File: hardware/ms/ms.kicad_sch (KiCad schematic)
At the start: 4 parts, among them U1 TP4056-42-ESOP8, U2 STM32G031G8Ux, U3 Opamp_Dual

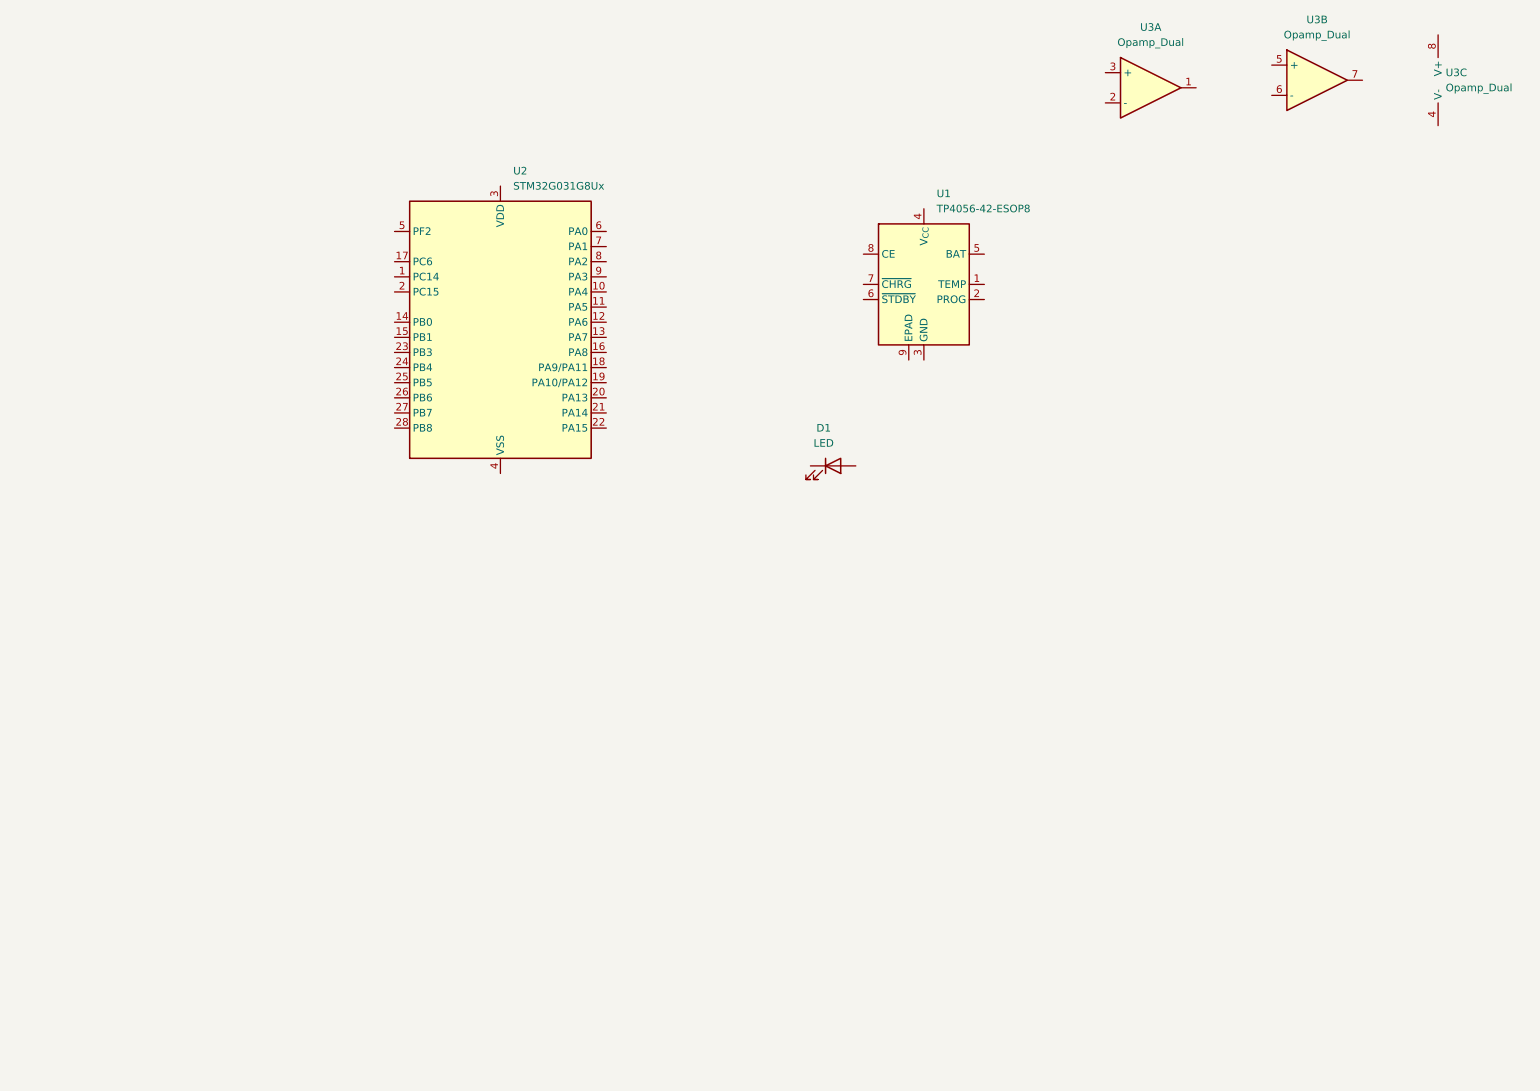
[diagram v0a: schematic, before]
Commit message: hardware update
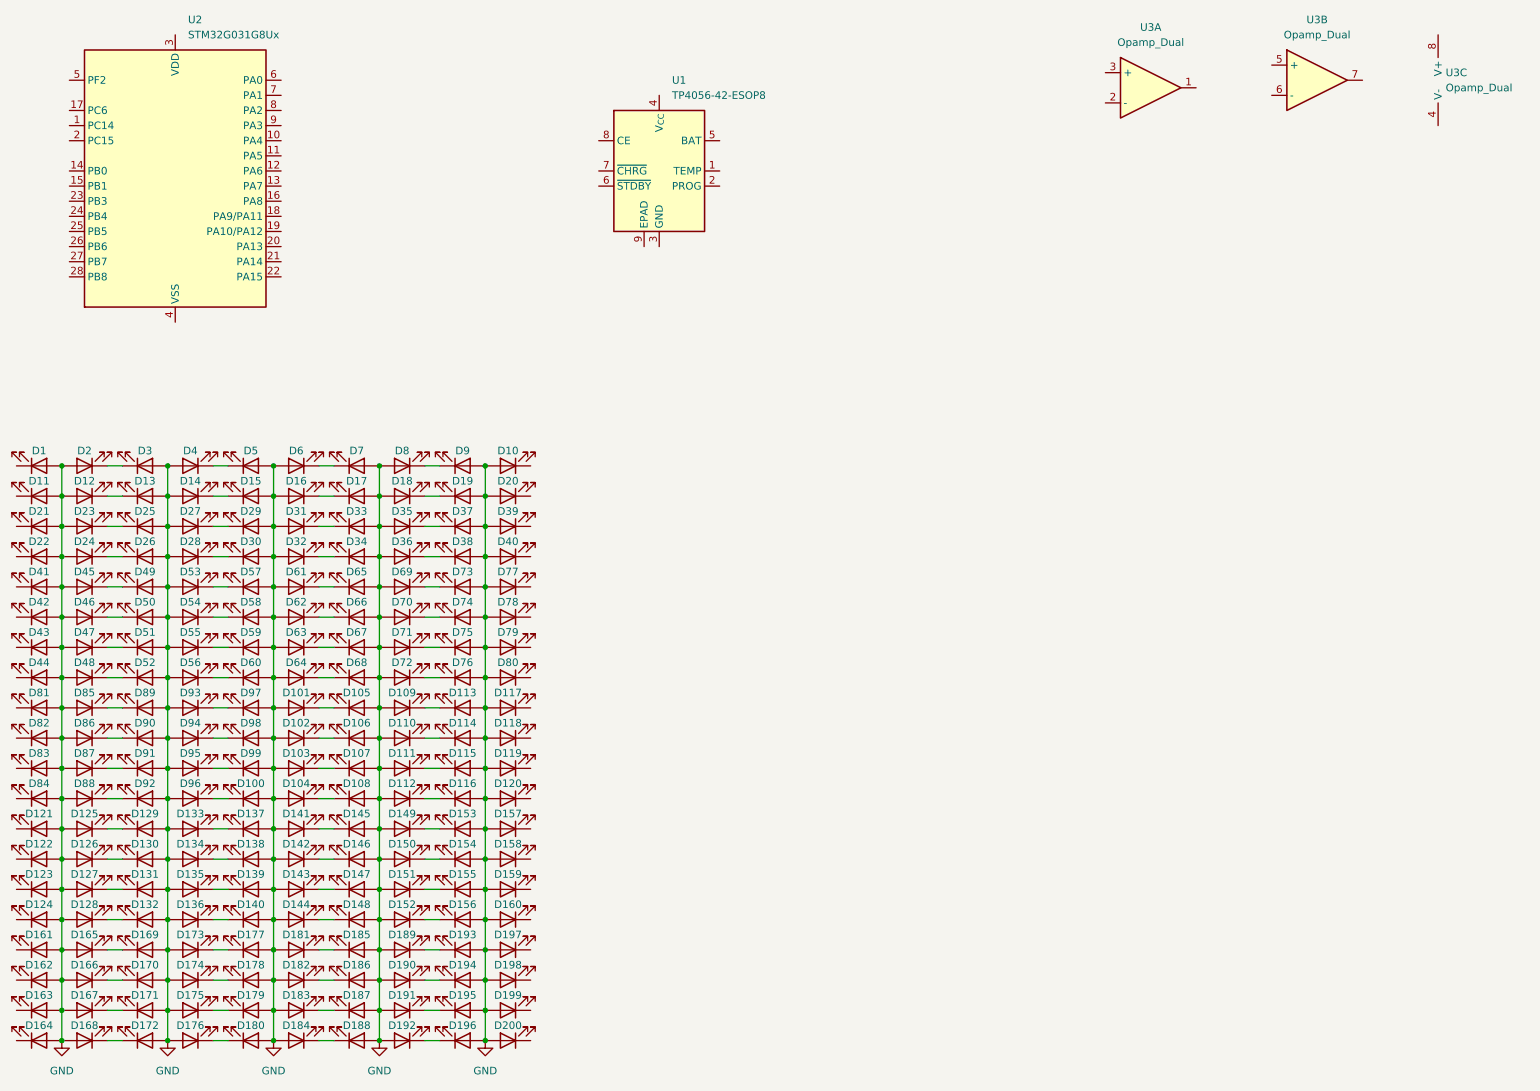
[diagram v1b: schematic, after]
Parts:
- added D10, D100, D101, D102, D103, D104, D105, D106, D107, D108, D109, D11, D110, D111, D112, D113, D114, D115, D116, D117, D118, D119, D12, D120, D121, D122, D123, D124, D125, D126, D127, D128, D129, D13, D130, D131, D132, D133, D134, D135, D136, D137, D138, D139, D14, D140, D141, D142, D143, D144, D145, D146, D147, D148, D149, D15, D150, D151, D152, D153, D154, D155, D156, D157, D158, D159, D16, D160, D161, D162, D163, D164, D165, D166, D167, D168, D169, D17, D170, D171, D172, D173, D174, D175, D176, D177, D178, D179, D18, D180, D181, D182, D183, D184, D185, D186, D187, D188, D189, D19, D190, D191, D192, D193, D194, D195, D196, D197, D198, D199, D2, D20, D200, D21, D22, D23, D24, D25, D26, D27, D28, D29, D3, D30, D31, D32, D33, D34, D35, D36, D37, D38, D39, D4, D40, D41, D42, D43, D44, D45, D46, D47, D48, D49, D5, D50, D51, D52, D53, D54, D55, D56, D57, D58, D59, D6, D60, D61, D62, D63, D64, D65, D66, D67, D68, D69, D7, D70, D71, D72, D73, D74, D75, D76, D77, D78, D79, D8, D80, D81, D82, D83, D84, D85, D86, D87, D88, D89, D9, D90, D91, D92, D93, D94, D95, D96, D97, D98, D99: LED, Library:LED, symbol Device:LED
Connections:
- net GND: now reaches D1.2 (A)
- net GND: now also D10.2 (A), D100.2 (A), D101.2 (A), D102.2 (A), D103.2 (A), D104.2 (A), D105.2 (A), D106.2 (A), D107.2 (A), D108.2 (A), D109.2 (A), D11.2 (A), D110.2 (A), D111.2 (A), D112.2 (A), D113.2 (A), D114.2 (A), D115.2 (A), D116.2 (A), D117.2 (A), D118.2 (A), D119.2 (A), D12.2 (A), D120.2 (A), D121.2 (A), D122.2 (A), D123.2 (A), D124.2 (A), D125.2 (A), D126.2 (A), D127.2 (A), D128.2 (A), D129.2 (A), D13.2 (A), D130.2 (A), D131.2 (A), D132.2 (A), D133.2 (A), D134.2 (A), D135.2 (A), D136.2 (A), D137.2 (A), D138.2 (A), D139.2 (A), D14.2 (A), D140.2 (A), D141.2 (A), D142.2 (A), D143.2 (A), D144.2 (A), D145.2 (A), D146.2 (A), D147.2 (A), D148.2 (A), D149.2 (A), D15.2 (A), D150.2 (A), D151.2 (A), D152.2 (A), D153.2 (A), D154.2 (A), D155.2 (A), D156.2 (A), D157.2 (A), D158.2 (A), D159.2 (A), D16.2 (A), D160.2 (A), D161.2 (A), D162.2 (A), D163.2 (A), D164.2 (A), D165.2 (A), D166.2 (A), D167.2 (A), D168.2 (A), D169.2 (A), D17.2 (A), D170.2 (A), D171.2 (A), D172.2 (A), D173.2 (A), D174.2 (A), D175.2 (A), D176.2 (A), D177.2 (A), D178.2 (A), D179.2 (A), D18.2 (A), D180.2 (A), D181.2 (A), D182.2 (A), D183.2 (A), D184.2 (A), D185.2 (A), D186.2 (A), D187.2 (A), D188.2 (A), D189.2 (A), D19.2 (A), D190.2 (A), D191.2 (A), D192.2 (A), D193.2 (A), D194.2 (A), D195.2 (A), D196.2 (A), D197.2 (A), D198.2 (A), D199.2 (A), D2.2 (A), D20.2 (A), D200.2 (A), D21.2 (A), D22.2 (A), D23.2 (A), D24.2 (A), D25.2 (A), D26.2 (A), D27.2 (A), D28.2 (A), D29.2 (A), D3.2 (A), D30.2 (A), D31.2 (A), D32.2 (A), D33.2 (A), D34.2 (A), D35.2 (A), D36.2 (A), D37.2 (A), D38.2 (A), D39.2 (A), D4.2 (A), D40.2 (A), D41.2 (A), D42.2 (A), D43.2 (A), D44.2 (A), D45.2 (A), D46.2 (A), D47.2 (A), D48.2 (A), D49.2 (A), D5.2 (A), D50.2 (A), D51.2 (A), D52.2 (A), D53.2 (A), D54.2 (A), D55.2 (A), D56.2 (A), D57.2 (A), D58.2 (A), D59.2 (A), D6.2 (A), D60.2 (A), D61.2 (A), D62.2 (A), D63.2 (A), D64.2 (A), D65.2 (A), D66.2 (A), D67.2 (A), D68.2 (A), D69.2 (A), D7.2 (A), D70.2 (A), D71.2 (A), D72.2 (A), D73.2 (A), D74.2 (A), D75.2 (A), D76.2 (A), D77.2 (A), D78.2 (A), D79.2 (A), D8.2 (A), D80.2 (A), D81.2 (A), D82.2 (A), D83.2 (A), D84.2 (A), D85.2 (A), D86.2 (A), D87.2 (A), D88.2 (A), D89.2 (A), D9.2 (A), D90.2 (A), D91.2 (A), D92.2 (A), D93.2 (A), D94.2 (A), D95.2 (A), D96.2 (A), D97.2 (A), D98.2 (A), D99.2 (A)
- new net: D142.1 (K), D146.1 (K)
- new net: D64.1 (K), D68.1 (K)
- new net: D167.1 (K), D171.1 (K)
- new net: D35.1 (K), D37.1 (K)
- new net: D152.1 (K), D156.1 (K)
- new net: D87.1 (K), D91.1 (K)
- new net: D62.1 (K), D66.1 (K)
- new net: D173.1 (K), D177.1 (K)
- new net: D23.1 (K), D25.1 (K)
- new net: D63.1 (K), D67.1 (K)
- new net: D71.1 (K), D75.1 (K)
- new net: D8.1 (K), D9.1 (K)
- new net: D135.1 (K), D139.1 (K)
- new net: D184.1 (K), D188.1 (K)
- new net: D168.1 (K), D172.1 (K)
- new net: D166.1 (K), D170.1 (K)
- new net: D88.1 (K), D92.1 (K)
- new net: D12.1 (K), D13.1 (K)
- new net: D141.1 (K), D145.1 (K)
- new net: D61.1 (K), D65.1 (K)
- new net: D2.1 (K), D3.1 (K)
- new net: D36.1 (K), D38.1 (K)
- new net: D144.1 (K), D148.1 (K)
- new net: D175.1 (K), D179.1 (K)
- new net: D95.1 (K), D99.1 (K)
- new net: D190.1 (K), D194.1 (K)
- new net: D191.1 (K), D195.1 (K)
- new net: D103.1 (K), D107.1 (K)
- new net: D100.1 (K), D96.1 (K)
- new net: D176.1 (K), D180.1 (K)
- new net: D14.1 (K), D15.1 (K)
- new net: D27.1 (K), D29.1 (K)
- new net: D109.1 (K), D113.1 (K)
- new net: D93.1 (K), D97.1 (K)
- new net: D125.1 (K), D129.1 (K)
- new net: D104.1 (K), D108.1 (K)
- new net: D31.1 (K), D33.1 (K)
- new net: D182.1 (K), D186.1 (K)
- new net: D181.1 (K), D185.1 (K)
- new net: D56.1 (K), D60.1 (K)
- new net: D189.1 (K), D193.1 (K)
- new net: D24.1 (K), D26.1 (K)
- new net: D111.1 (K), D115.1 (K)
- new net: D110.1 (K), D114.1 (K)
- new net: D86.1 (K), D90.1 (K)
- new net: D6.1 (K), D7.1 (K)
- new net: D165.1 (K), D169.1 (K)
- new net: D112.1 (K), D116.1 (K)
- new net: D126.1 (K), D130.1 (K)
- new net: D150.1 (K), D154.1 (K)
- new net: D151.1 (K), D155.1 (K)
- new net: D69.1 (K), D73.1 (K)
- new net: D70.1 (K), D74.1 (K)
- new net: D85.1 (K), D89.1 (K)
- new net: D183.1 (K), D187.1 (K)
- new net: D47.1 (K), D51.1 (K)
- new net: D46.1 (K), D50.1 (K)
- new net: D101.1 (K), D105.1 (K)
- new net: D127.1 (K), D131.1 (K)
- new net: D136.1 (K), D140.1 (K)
- new net: D133.1 (K), D137.1 (K)
- new net: D53.1 (K), D57.1 (K)
- new net: D18.1 (K), D19.1 (K)
- new net: D174.1 (K), D178.1 (K)
- new net: D4.1 (K), D5.1 (K)
- new net: D94.1 (K), D98.1 (K)
- new net: D102.1 (K), D106.1 (K)
- new net: D28.1 (K), D30.1 (K)
- new net: D134.1 (K), D138.1 (K)
- new net: D143.1 (K), D147.1 (K)
- new net: D45.1 (K), D49.1 (K)
- new net: D128.1 (K), D132.1 (K)
- new net: D32.1 (K), D34.1 (K)
- new net: D149.1 (K), D153.1 (K)
- new net: D55.1 (K), D59.1 (K)
- new net: D16.1 (K), D17.1 (K)
- new net: D48.1 (K), D52.1 (K)
- new net: D54.1 (K), D58.1 (K)
- new net: D72.1 (K), D76.1 (K)
- new net: D192.1 (K), D196.1 (K)
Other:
- moved on the sheet: U1, U2

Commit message: hw update for new design
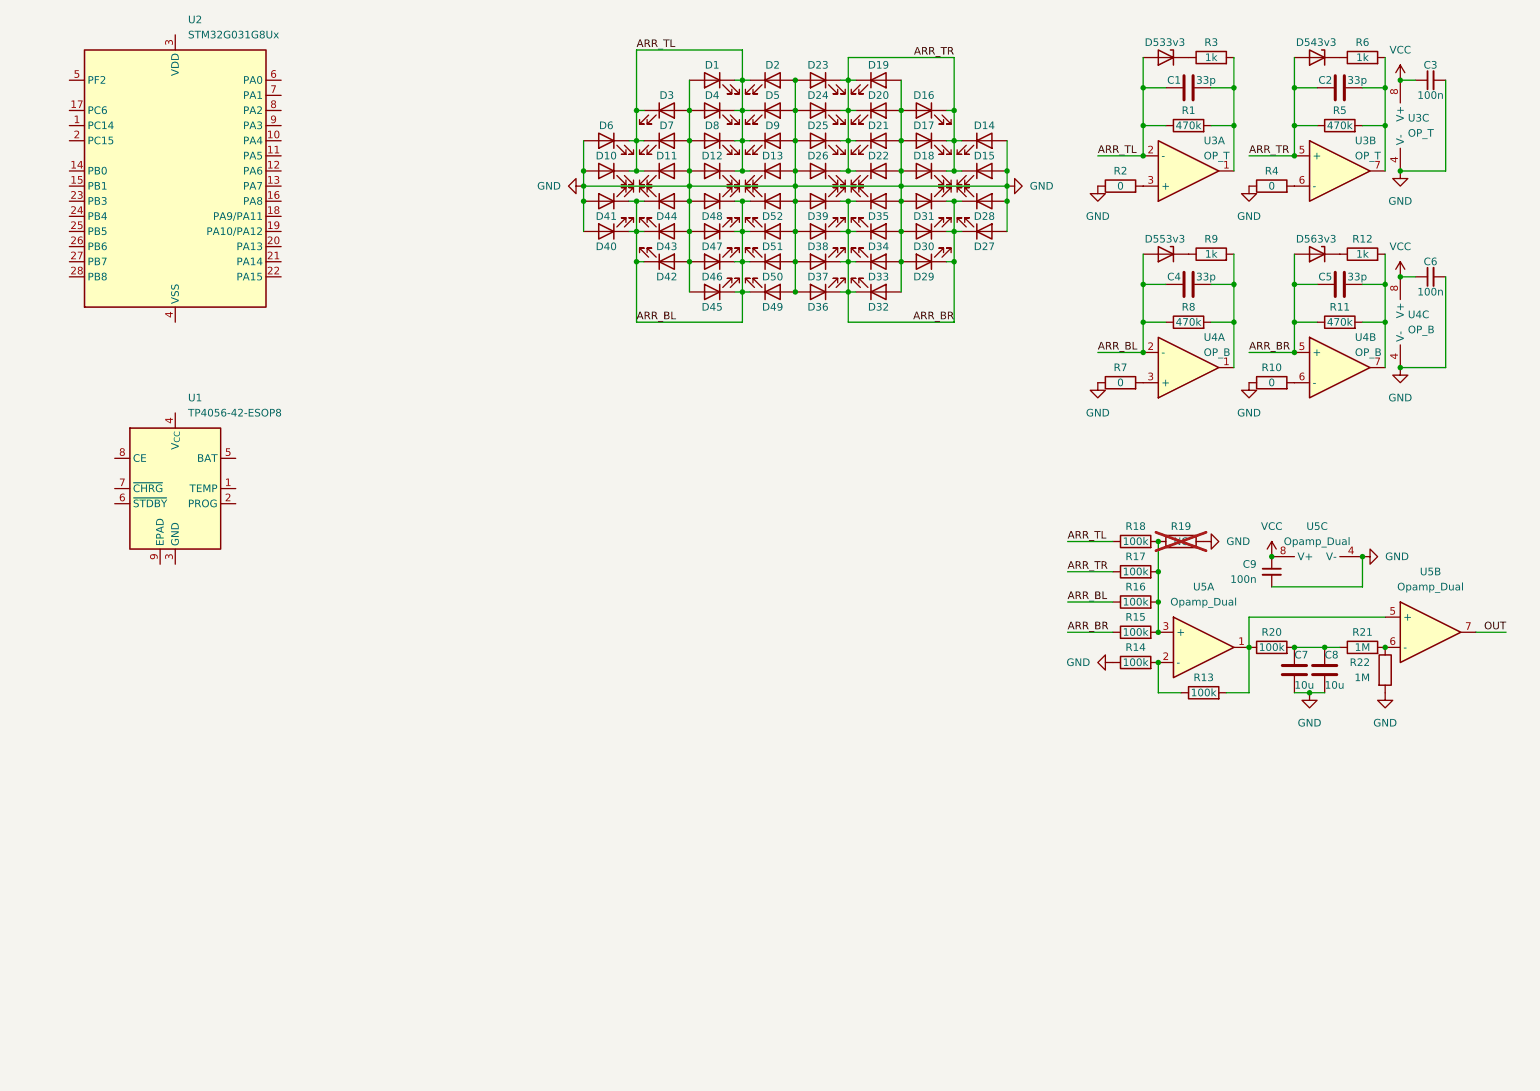
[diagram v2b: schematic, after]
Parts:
- removed D100, D101, D102, D103, D104, D105, D106, D107, D108, D109, D110, D111, D112, D113, D114, D115, D116, D117, D118, D119, D120, D121, D122, D123, D124, D125, D126, D127, D128, D129, D130, D131, D132, D133, D134, D135, D136, D137, D138, D139, D140, D141, D142, D143, D144, D145, D146, D147, D148, D149, D150, D151, D152, D153, D154, D155, D156, D157, D158, D159, D160, D161, D162, D163, D164, D165, D166, D167, D168, D169, D170, D171, D172, D173, D174, D175, D176, D177, D178, D179, D180, D181, D182, D183, D184, D185, D186, D187, D188, D189, D190, D191, D192, D193, D194, D195, D196, D197, D198, D199, D200, D53, D54, D55, D56, D57, D58, D59, D60, D61, D62, D63, D64, D65, D66, D67, D68, D69, D70, D71, D72, D73, D74, D75, D76, D77, D78, D79, D80, D81, D82, D83, D84, D85, D86, D87, D88, D89, D90, D91, D92, D93, D94, D95, D96, D97, D98, D99: LED, Library:LED, symbol Device:LED
- added C1, C2, C4, C5: 33p, symbol Device:C
- added C3, C6, C9: 100n, symbol Device:C_Small
- added C7, C8: 10u, symbol Device:C
- added D53, D54, D55, D56: 3v3, symbol Device:D_Zener
- added R1, R11, R5, R8: 470k, symbol Device:R
- added R10, R2, R4, R7: 0, symbol Device:R
- added R12, R3, R6, R9: 1k, symbol Device:R
- added R13, R14, R15, R16, R17, R18, R20: 100k, symbol Device:R
- added R19: NC, symbol Device:R
- added R21, R22: 1M, symbol Device:R
- added U4: OP_B, Package_SO:SOIC-8_3.9x4.9mm_P1.27mm, symbol Device:Opamp_Dual
- added U5: Opamp_Dual, Package_SO:SOIC-8_3.9x4.9mm_P1.27mm, symbol Device:Opamp_Dual
- D1, D10, D11, D12, D13, D14, D15, D16, D17, D18, D19, D2, D20, D21, D22, D23, D24, D25, D26, D27, D28, D29, D3, D30, D31, D32, D33, D34, D35, D36, D37, D38, D39, D4, D40, D41, D42, D43, D44, D45, D46, D47, D48, D49, D5, D50, D51, D52, D6, D7, D8, D9: footprint Library:LED -> LED_THT:LED_D5.0mm_Clear
- U3: value Opamp_Dual -> OP_T
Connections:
- net GND: now also U3.4 (V-), C3.2, C6.2, C7.2, C8.2, C9.2, R10.1, R14.1, R19.2, R2.1, R22.2, R4.1, R7.1, U4.4 (V-), U5.4 (V-)
- net ARR_BR: now reaches D35.1 (K), D37.1 (K)
- net ARR_BR: now also D27.1 (K), D28.1 (K), D29.1 (K), D30.1 (K), D31.1 (K), D32.1 (K), D33.1 (K), D34.1 (K), D36.1 (K), D38.1 (K), D39.1 (K), C5.1, D56.2 (A), R11.1, R15.1, U4.5 (+)
- net ARR_TR: now reaches D23.1 (K), D25.1 (K)
- net ARR_TR: now also D14.1 (K), D15.1 (K), D16.1 (K), D17.1 (K), D18.1 (K), D19.1 (K), D20.1 (K), D21.1 (K), D22.1 (K), D24.1 (K), D26.1 (K), U3.5 (+), C2.1, D54.2 (A), R17.1, R5.1
- net ARR_TL: now reaches D8.1 (K), D9.1 (K)
- net ARR_TL: now also D1.1 (K), D10.1 (K), D11.1 (K), D12.1 (K), D13.1 (K), D2.1 (K), D3.1 (K), D4.1 (K), D5.1 (K), D6.1 (K), D7.1 (K), U3.2 (-), C1.1, D53.2 (A), R1.1, R18.1
- net ARR_BL: now reaches D42.1 (K)
- net ARR_BL: now also D40.1 (K), D41.1 (K), D43.1 (K), D44.1 (K), D45.1 (K), D46.1 (K), D47.1 (K), D48.1 (K), D49.1 (K), D50.1 (K), D51.1 (K), D52.1 (K), C4.1, D55.2 (A), R16.1, R8.1, U4.2 (-)
- net VCC: now reaches U3.8 (V+)
- net VCC: now also C3.1, C6.1, C9.1, U4.8 (V+), U5.8 (V+)
- net at U3.6 (-): now also R4.2
- net at U3.7: now also C2.2, R5.2, R6.2
- net at U3.1: now also C1.2, R1.2, R3.2
- net at U3.3 (+): now also R2.2
- new net: R7.2, U4.3 (+)
- new net: R15.2, R16.2, R17.2, R18.2, R19.1, U5.3 (+)
- new net: R10.2, U4.6 (-)
- new net: R13.1, R14.2, U5.2 (-)
- new net: R13.2, R20.1, U5.1, U5.5 (+)
- new net: D55.1 (K), R9.1
- new net: C4.2, R8.2, R9.2, U4.1
- new net: R21.2, R22.1, U5.6 (-)
- new net: C7.1, C8.1, R20.2, R21.1
- new net: D53.1 (K), R3.1
- new net: C5.2, R11.2, R12.2, U4.7
- new net: D56.1 (K), R12.1
- new net: D54.1 (K), R6.1
- new net OUT: U5.7
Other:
- moved on the sheet: U1, U3A, U3B, U3C
